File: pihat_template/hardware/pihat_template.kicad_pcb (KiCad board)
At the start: 2 copper layers, 65 x 56.5 mm, 37 parts, among them P1 CONN_01X02, P2 CONN_01X02, P3 Raspberry_Pi_+_Conn, Q1 BSS138, U1 LM3489, U2 CAT24C32HU4I-GT3, U3 FDC5614P, U4 LM1117IMPX-ADJ, U5 DMMT5401

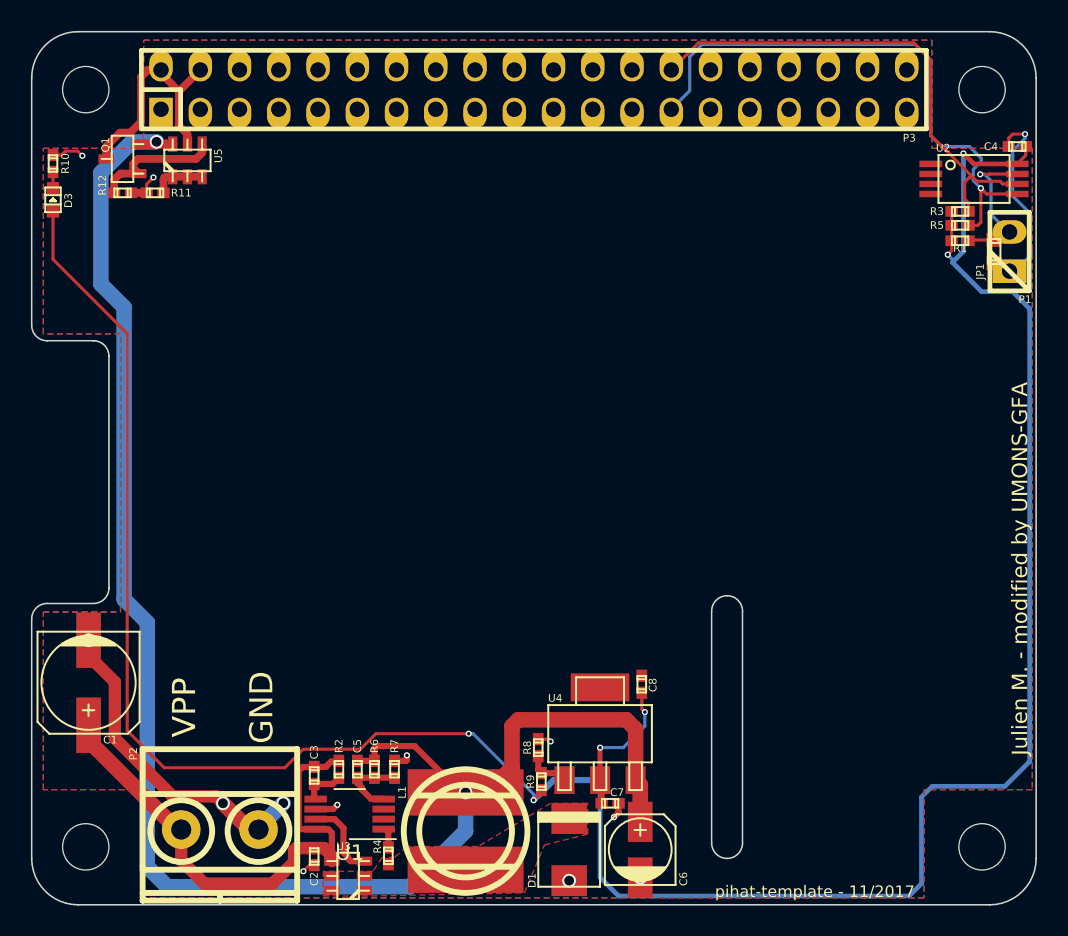
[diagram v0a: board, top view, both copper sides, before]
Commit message: updated vias for EuroCircuits standards
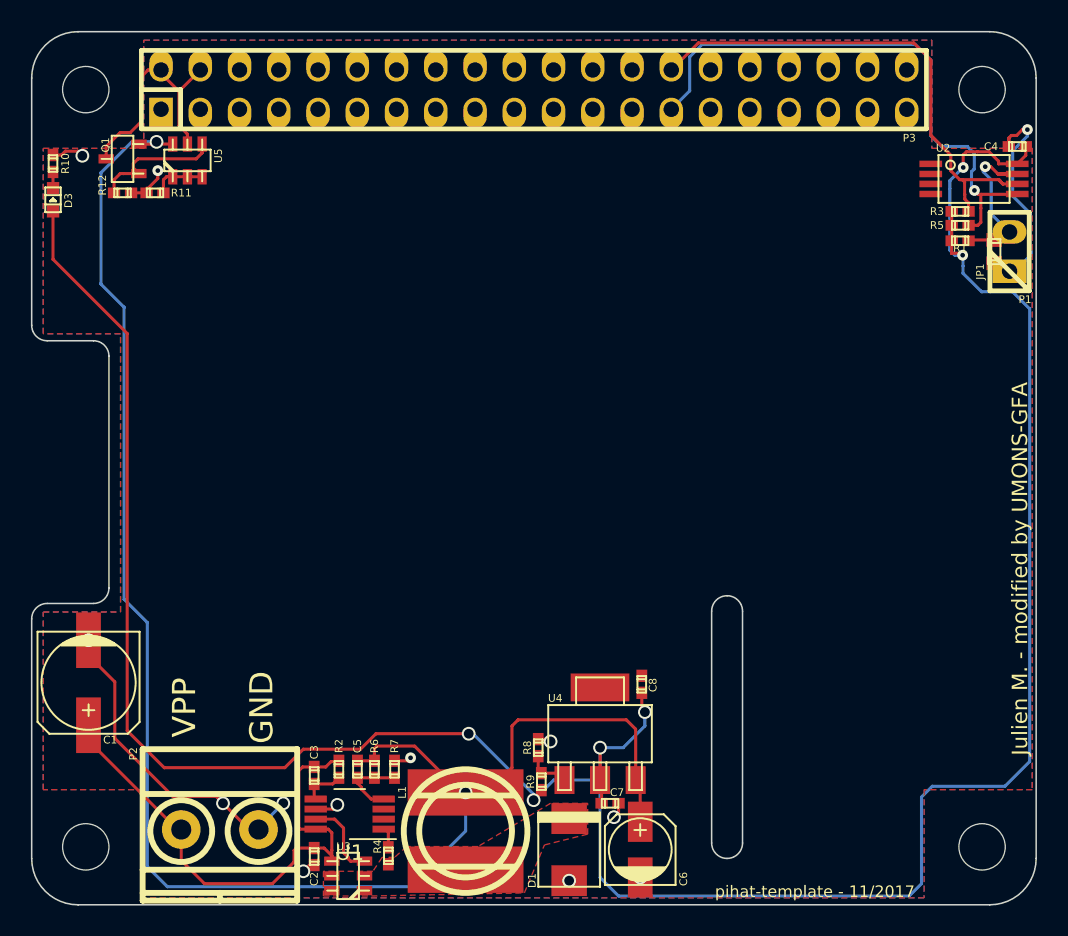
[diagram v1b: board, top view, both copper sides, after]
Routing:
- net GND: track 44.4 -> 46.7 mm
- net Net-(JP1-Pad1): track 10.0 -> 11.5 mm
- net +3V3: track 176.1 -> 176.7 mm
- net Net-(P3-Pad28): track 32.4 -> 32.9 mm
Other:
- rule via_min_drill: 0.16 -> 0.3
- rule via_min_size: 0.26 -> 0.7
